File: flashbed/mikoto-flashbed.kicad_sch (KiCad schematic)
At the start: 10 parts, among them J1 Conn_01x01, J2 Conn_01x01, J3 Conn_01x01, J4 Conn_01x01, J7 Conn_01x05, J8 Conn_01x01, SW1 TVBP06, U1 mikoto-pins

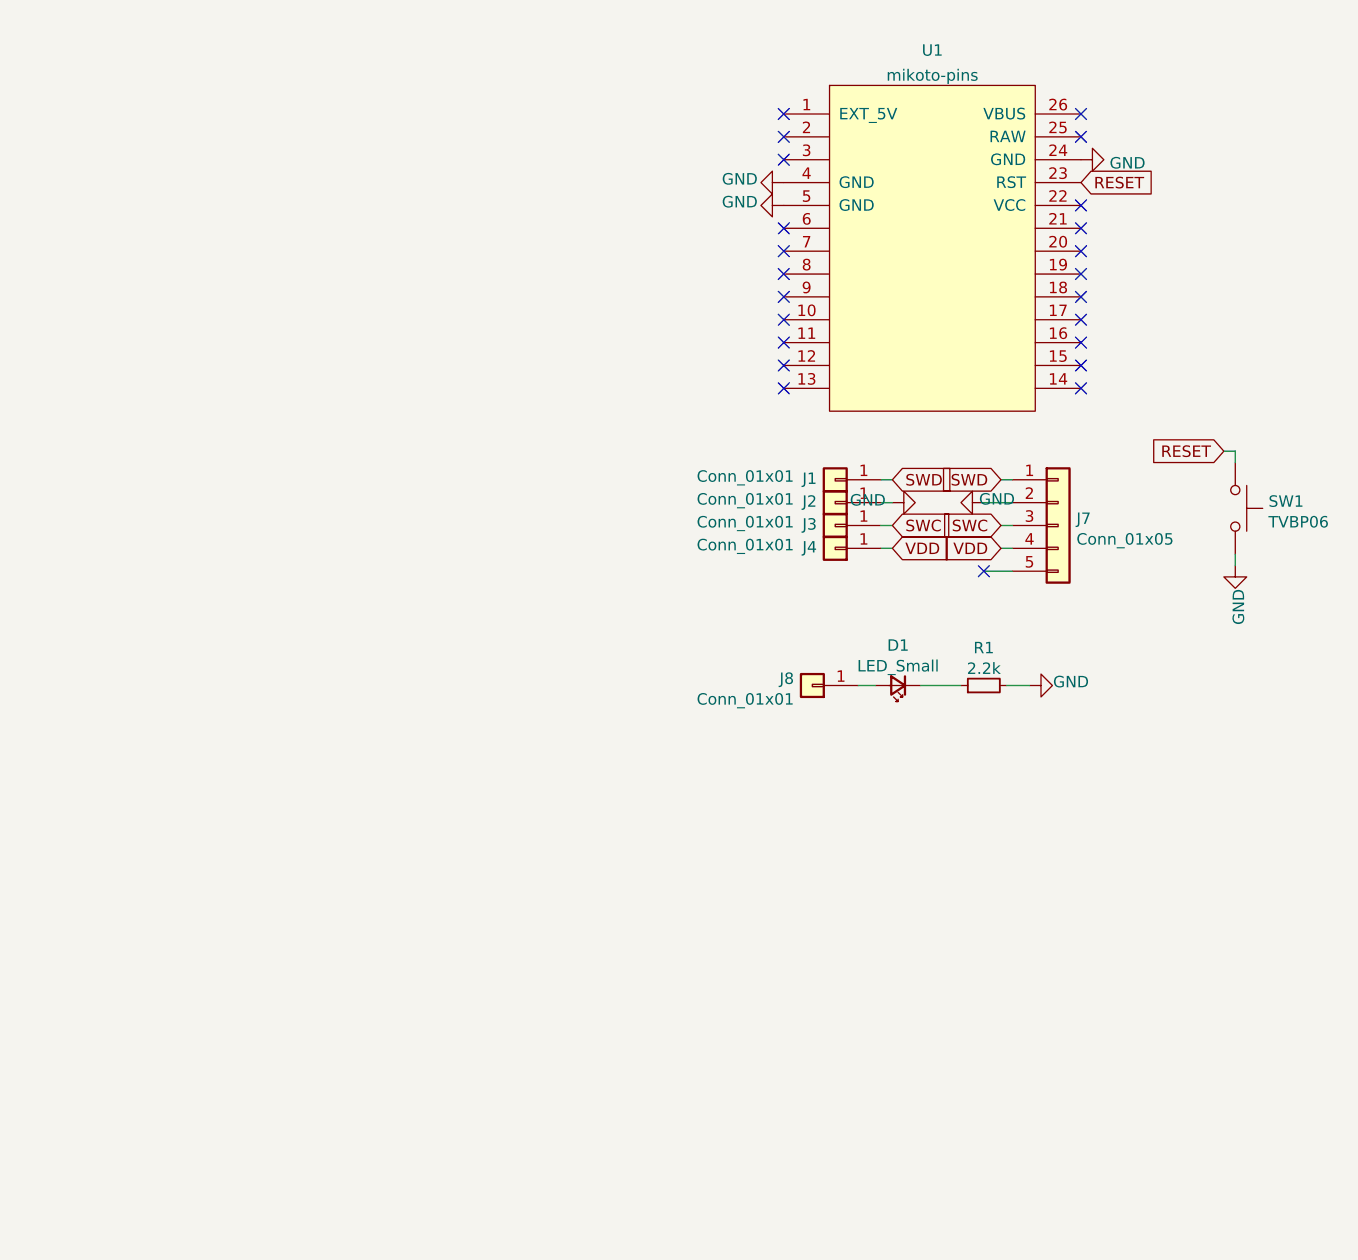
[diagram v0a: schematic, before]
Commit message: update flashbed
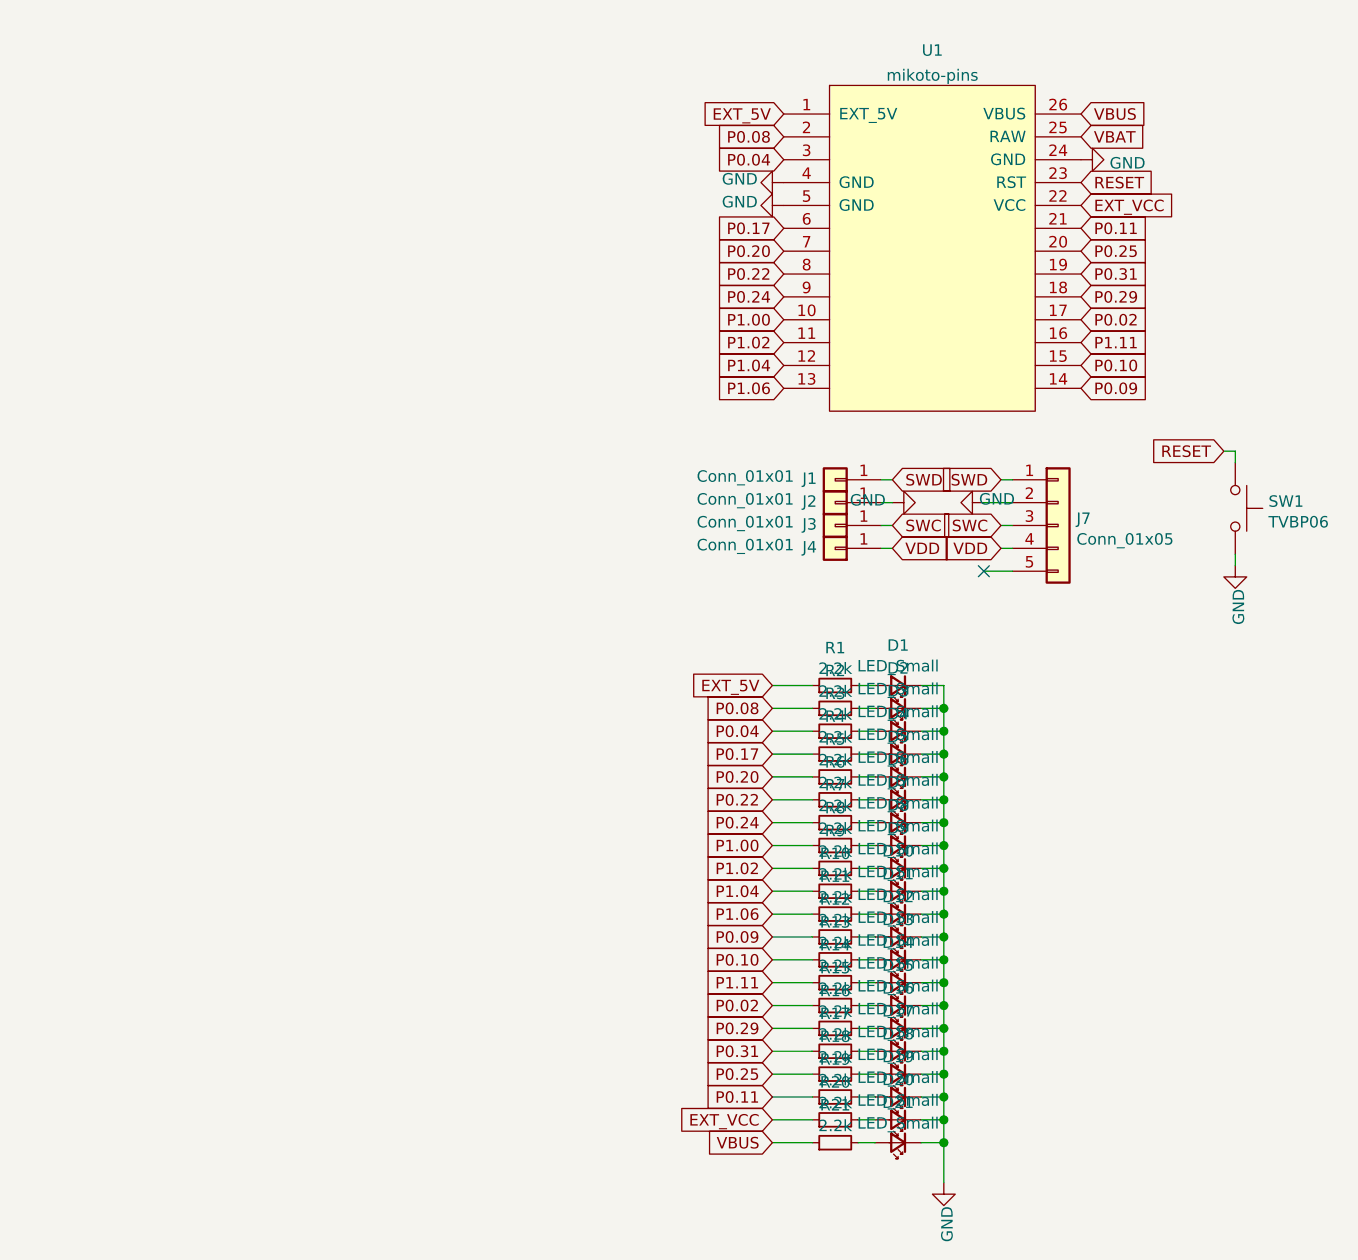
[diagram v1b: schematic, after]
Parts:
- removed J8: Conn_01x01, Connector_PinHeader_2.54mm:PinHeader_1x01_P2.54mm_Vertical, symbol Connector_Generic:Conn_01x01
- added D10, D11, D12, D13, D14, D15, D16, D17, D18, D19, D2, D20, D21, D3, D4, D5, D6, D7, D8, D9: LED_Small, footprints:LED_1206_3216M_Castellated-nosilk, symbol Device:LED_Small
- added R10, R11, R12, R13, R14, R15, R16, R17, R18, R19, R2, R20, R21, R3, R4, R5, R6, R7, R8, R9: 2.2k, Resistor_SMD:R_0805_2012Metric_Pad1.15x1.40mm_HandSolder, symbol Device:R_Small
- D1: footprint LED_SMD:LED_1206_3216Metric_Pad1.42x1.75mm_HandSolder -> footprints:LED_1206_3216M_Castellated-nosilk
- U1: footprint footprints:mikoto-pins -> footprints:mikoto-pins-bigger-holes
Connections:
- net GND: now also D1.1 (K), D10.1 (K), D11.1 (K), D12.1 (K), D13.1 (K), D14.1 (K), D15.1 (K), D16.1 (K), D17.1 (K), D18.1 (K), D19.1 (K), D2.1 (K), D20.1 (K), D21.1 (K), D3.1 (K), D4.1 (K), D5.1 (K), D6.1 (K), D7.1 (K), D8.1 (K), D9.1 (K); no longer R1.2
- net EXT_5V: now reaches U1.1 (EXT_5V)
- net EXT_5V: now also R1.1
- net P1.00: now reaches U1.10
- net P1.00: now also R8.1
- net P1.02: now reaches U1.11
- net P1.02: now also R9.1
- net P1.04: now reaches U1.12
- net P1.04: now also R10.1
- net P1.06: now reaches U1.13
- net P1.06: now also R11.1
- net P0.09: now reaches U1.14
- net P0.09: now also R12.1
- net P0.10: now reaches U1.15
- net P0.10: now also R13.1
- net P1.11: now reaches U1.16
- net P1.11: now also R14.1
- net P0.02: now reaches U1.17
- net P0.02: now also R15.1
- net P0.29: now reaches U1.18
- net P0.29: now also R16.1
- net P0.31: now reaches U1.19
- net P0.31: now also R17.1
- net P0.08: now reaches U1.2
- net P0.08: now also R2.1
- net P0.25: now reaches U1.20
- net P0.25: now also R18.1
- net P0.11: now reaches U1.21
- net P0.11: now also R19.1
- net EXT_VCC: now reaches U1.22 (VCC)
- net EXT_VCC: now also R20.1
- net VBAT: now reaches U1.25 (RAW)
- net VBUS: now reaches U1.26 (VBUS)
- net VBUS: now also R21.1
- net P0.04: now reaches U1.3
- net P0.04: now also R3.1
- net P0.17: now reaches U1.6
- net P0.17: now also R4.1
- net P0.20: now reaches U1.7
- net P0.20: now also R5.1
- net P0.22: now reaches U1.8
- net P0.22: now also R6.1
- net P0.24: now reaches U1.9
- net P0.24: now also R7.1
- net at D1.2 (A): now also R1.2
- new net: D10.2 (A), R10.2
- new net: D16.2 (A), R16.2
- new net: D11.2 (A), R11.2
- new net: D4.2 (A), R4.2
- new net: D12.2 (A), R12.2
- new net: D14.2 (A), R14.2
- new net: D3.2 (A), R3.2
- new net: D7.2 (A), R7.2
- new net: D2.2 (A), R2.2
- new net: D18.2 (A), R18.2
- new net: D5.2 (A), R5.2
- new net: D6.2 (A), R6.2
- new net: D15.2 (A), R15.2
- new net: D17.2 (A), R17.2
- new net: D13.2 (A), R13.2
- new net: D21.2 (A), R21.2
- new net: D8.2 (A), R8.2
- new net: D20.2 (A), R20.2
- new net: D9.2 (A), R9.2
- new net: D19.2 (A), R19.2
- no-connect marks 23 -> 1
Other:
- moved on the sheet: R1

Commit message: some nonsense with the flashbed
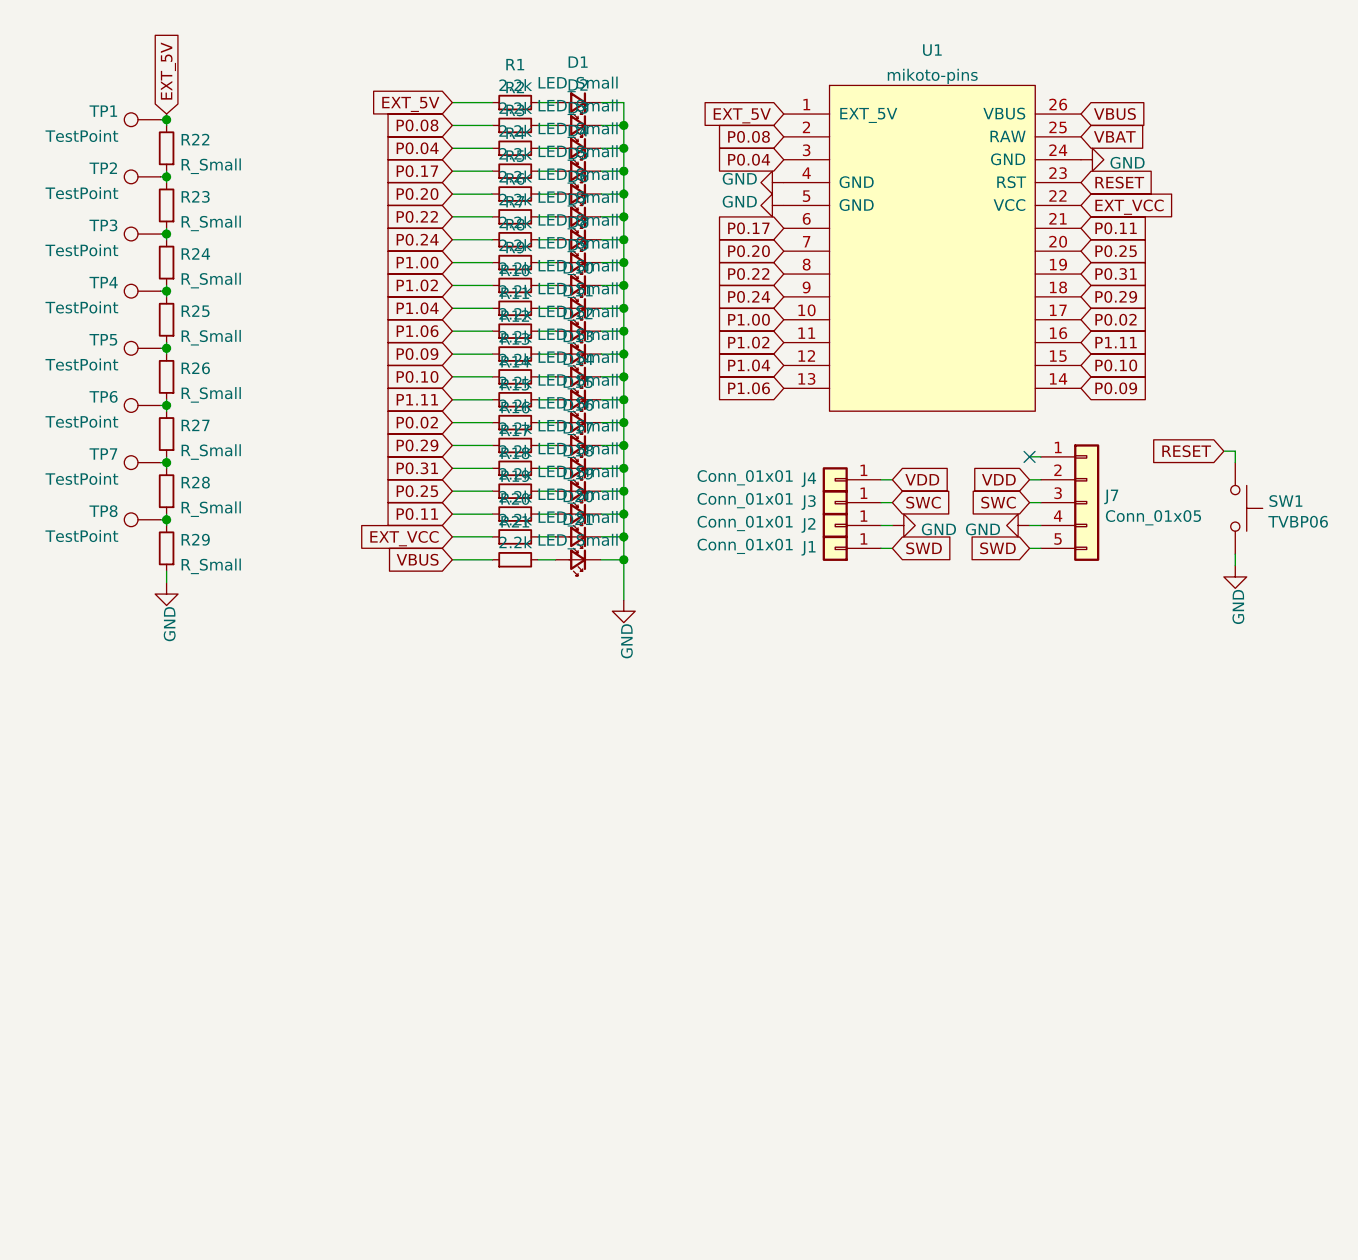
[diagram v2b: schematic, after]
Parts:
- added R22, R23, R24, R25, R26, R27, R28, R29: R_Small, Resistor_SMD:R_0201_0603Metric, symbol Device:R_Small
- added TP1, TP2, TP3, TP4, TP5, TP6, TP7, TP8: TestPoint, footprints:TestPoint_Pad_D1.0mm-nosilk, symbol Connector:TestPoint
- J7: footprint Connector_PinHeader_2.54mm:PinHeader_1x05_P2.54mm_Vertical -> Connector_PinHeader_2.54mm:PinHeader_1x05_P2.54mm_Horizontal
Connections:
- net EXT_5V: now also R22.2, TP1.1
- net GND: now also J7.4 (Pin_4), R29.1; no longer J7.2 (Pin_2)
- net SWD: now also J7.5 (Pin_5); no longer J7.1 (Pin_1)
- net VDD: now also J7.2 (Pin_2); no longer J7.4 (Pin_4)
- new net: R22.1, R23.2, TP2.1
- new net: R25.1, R26.2, TP5.1
- new net: R27.1, R28.2, TP7.1
- new net: R28.1, R29.2, TP8.1
- new net: R24.1, R25.2, TP4.1
- new net: R23.1, R24.2, TP3.1
- new net: R26.1, R27.2, TP6.1
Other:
- moved on the sheet: D1, D10, D11, D12, D13, D14, D15, D16, D17, D18, D19, D2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
